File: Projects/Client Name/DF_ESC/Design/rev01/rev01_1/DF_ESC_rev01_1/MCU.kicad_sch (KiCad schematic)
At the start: 38 parts, among them U1 STM32F405RGTx

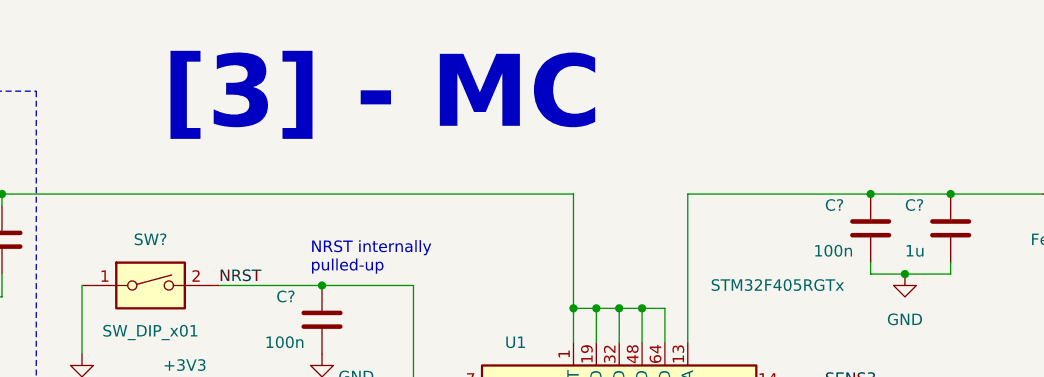
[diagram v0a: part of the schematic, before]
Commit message: Update MCU.kicad_sch
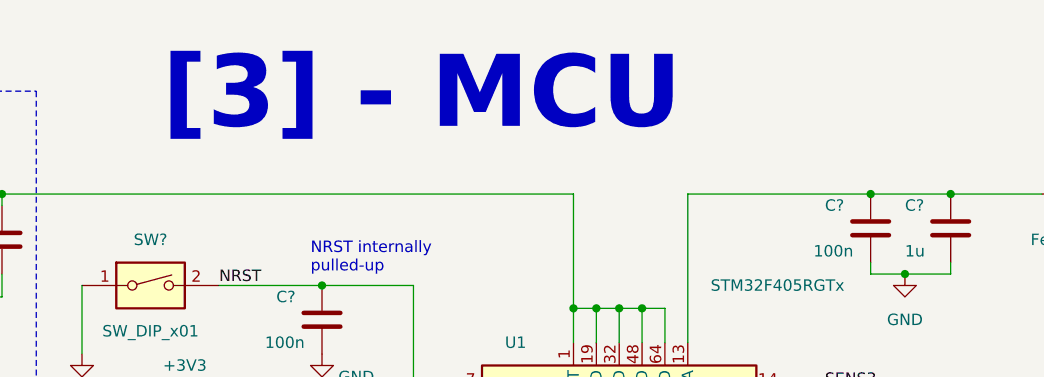
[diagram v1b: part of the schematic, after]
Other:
- note added: "[3] - MCU"
- note removed: "[3] - MC"
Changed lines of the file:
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@@
     )
   )
-  (text "[3] - MC" (at 123.19 31.75 0)
+  (text "[3] - MCU" (at 123.19 31.75 0)
     (effects (font (size 8 8) (thickness 1.6) bold) (justify left bottom))
   )
